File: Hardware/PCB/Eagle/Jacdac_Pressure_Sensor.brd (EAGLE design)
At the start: 27.9 x 27.9 mm, 29 parts, among them J1 JACDAC_EDGE_CONN-INNIE, J2 SWD-ADAPTER-, U1 NCP114ASN330T1G, U2 STM32F042F6P6, U3 LPS33HWTR, U4 BAT54S,235

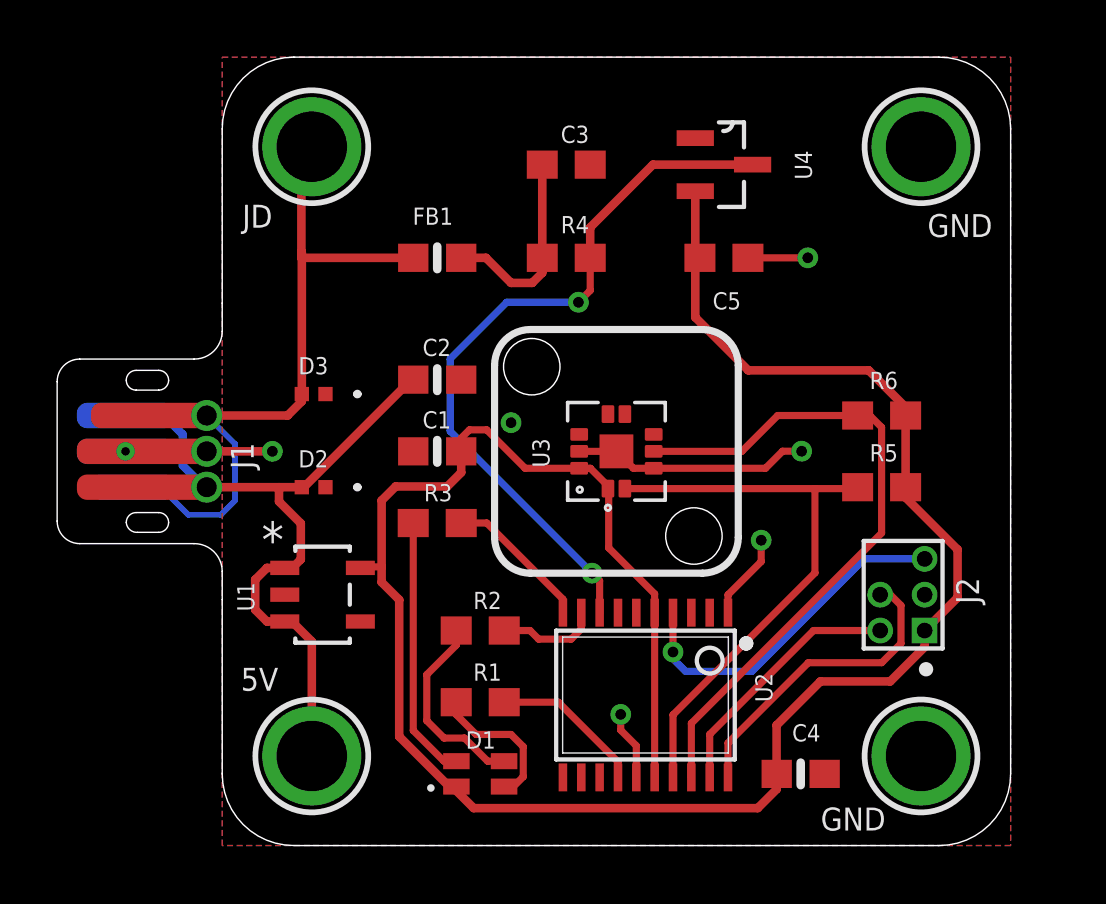
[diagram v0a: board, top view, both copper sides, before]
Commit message: Added version 1.0
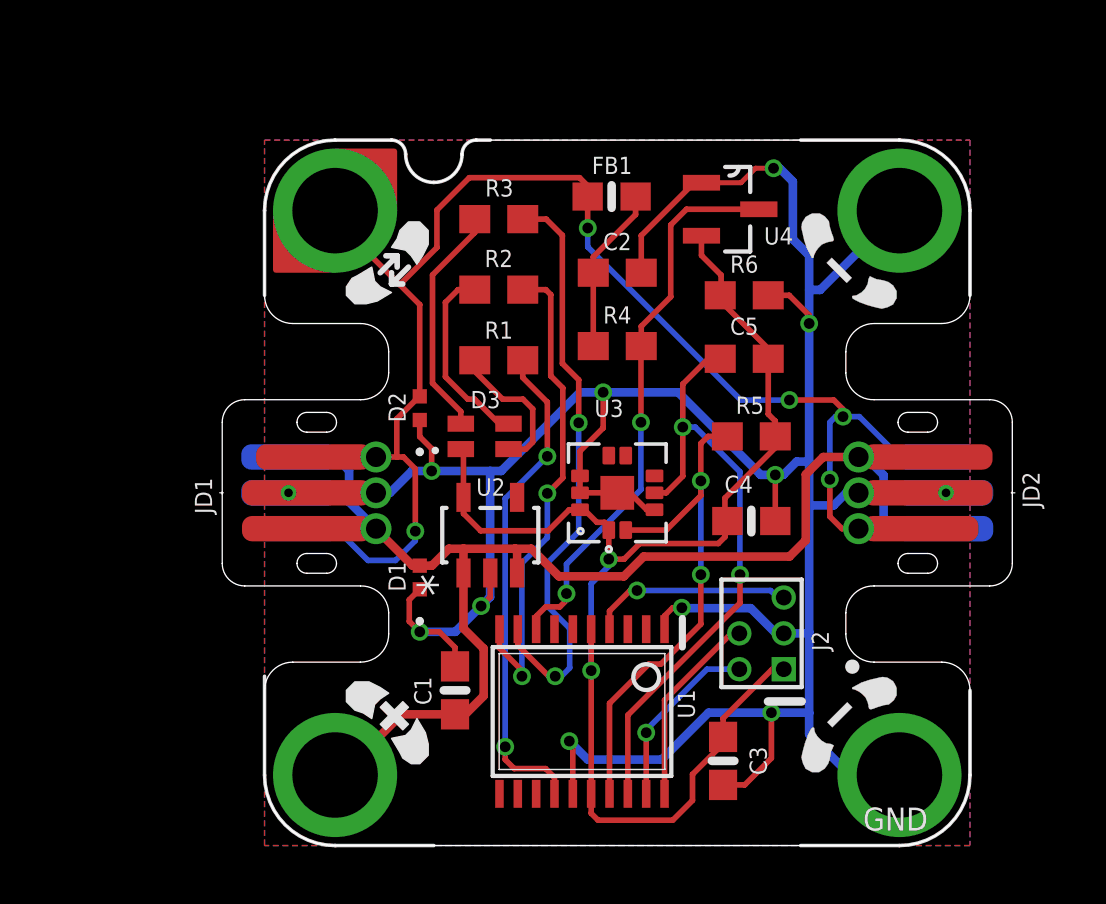
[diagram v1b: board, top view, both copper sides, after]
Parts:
- removed H1, H2, H3, H4: MOUNTINGHOLE2.5, milador:MOUNTINGHOLE_2.5_PLATED
- removed J1: JACDAC_EDGE_CONN-INNIE, Jacdac:JACDAC-EDGE-CONN-INNIE
- removed LABEL2: JACDAC-DEVICE-PS, milador:JACDAC-PRESSURE-SENSOR
- removed LABEL3: MILADOR-LOGO-, milador:MILADOR_LOGO1
- removed U$1: JACDAC-DEVICE-LPS33HW, milador:JACDAC-LPS33HW
- added J3: 5V, milador:M3-HOLE-PWR-OUTL
- added J4: DATA, milador:M3-HOLE-DATA-NOTCH
- added J5, J6: GND, milador:M3-HOLE-GND
- added JD1, JD2: JACDAC-EDGE-OUTIE, milador:JD-EDGE-OUTIE
- added LABEL_JACDAC_PS: MILADOR-JACDAC-DEVICE-PS, milador:JACDAC-PRESSURE-SENSOR
- added LABEL_LPS33HW: MILADOR-JACDAC-DEVICE-LPS33HW, milador:JACDAC-LPS33HW
- added LABEL_MILADOR: MILADOR-LOGO-, milador:MILADOR_LOGO1
- added LABEL_QR_CODE: MILADOR-QR-CODE-JACDAC-GITHUB-PS, milador:MILADOR_QR_JACDAC_PS
- C1: value 0.1uF -> 1uF
- C2: value 1uF -> 33pF; device milador_SMD:0603-NO -> milador_SMD:0603
- C3: value 33pF -> 1uF; device milador_SMD:0603 -> milador_SMD:0603-NO
- C4: value 1uF -> 0.1uF
- D1: value LED-HSMF-C114 -> DIODE-ZENER-AA-RCLAMP0521PATCT; device milador_SMD:DIOSC160X150X35-4N -> milador_SMD:DIODE-ZENER-0402
- D2: value RCLAMP0521PATCT -> DIODE-ZENER-AA-RCLAMP0521PATCT
- D3: value RCLAMP0521PATCT -> LED-HSMF-C114; device milador_SMD:DIODE-ZENER-0402 -> milador_SMD:DIOSC160X150X35-4N
- MMC_LOGO: value MMC_LOGO-SM -> MMC_LOGO-XSM; device MMC Eagle:MMC_SMALL_LOGO -> MMC Eagle:MMC_X-SMALL_LOGO
- U1: value NCP114ASN330T1G -> STM32F042F6P6; device milador_SMD:TSOP-5_ONS -> milador_SMD:TSSOP20
- U2: value STM32F042F6P6 -> NCP114ASN330T1G; device milador_SMD:TSSOP20 -> milador_SMD:TSOP-5_ONS
- moved C3 21.8 mm to (17.8, 3.00), turned to 270 degrees
- moved R1 12.1 mm to (9.80, 17.2)
- moved R2 12.1 mm to (9.80, 19.7)
- moved R3 11.0 mm to (9.80, 22.2)
- moved U1 10.1 mm to (12.8, 4.75), turned to 180 degrees
- moved MMC_LOGO 9.48 mm to (12.0, 4.50), turned to 0 degrees
- moved C4 9.13 mm to (18.8, 11.5)
- moved C1 8.49 mm to (8.25, 5.50), turned to 90 degrees
- moved U2 7.90 mm to (9.50, 11.0), turned to 90 degrees
- moved C2 7.42 mm to (14.0, 20.3)
- moved D1 7.28 mm to (7.00, 9.50), turned to 90 degrees
- moved FB1 6.55 mm to (13.8, 23.0)
- moved D3 6.24 mm to (9.30, 14.5), turned to 0 degrees
- moved R6 5.27 mm to (18.5, 17.2)
- moved J2 5.18 mm to (19.9, 6.25)
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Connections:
- net +3V3: now also C3.1, D3.1, U1.16; no longer C1.1, D1.1, U2.16
- net GND: now also D1.1, J5.H, J6.H, JD1.2, JD1.5, JD1.P$2, JD1.P$4, JD2.2, JD2.5, JD2.P$2, JD2.P$4, U1.1, U1.15, U2.2; no longer D3.1, H3.P$1, H4.P$1, J1.GND1, J1.GND2, J1.GND3, J1.GND4, U1.2, U2.1, U2.15
- net JD_DATA: now also U1.8; no longer U2.8
- net J_DATA: now also D2.2, J4.H, JD1.1, JD1.6, JD1.P$3, JD2.1, JD2.6, JD2.P$3; no longer D3.2, H2.P$1, J1.JD1, J1.JD2, J1.JD3
- net N$1: now also D3.4; no longer D1.4
- net N$2: now also D3.3; no longer D1.3
- net N$3: now also D3.2; no longer D1.2
- net N$4: now also C2.1; no longer C3.1
- net RESET: now also U1.4; no longer U2.4
- net RGB_B: now also U1.14; no longer U2.14
- net RGB_G: now also U1.10; no longer U2.9
- net RGB_R: now also U1.9; no longer U2.10
- net SCL: now also U1.17; no longer U2.17
- net SDA: now also U1.18; no longer U2.18
- net SWCLK: now also U1.20; no longer U2.20
- net SWDIO: now also U1.19; no longer U2.19
- net VCC: now also C1.1, D1.2, J3.H, JD1.3, JD1.4, JD1.P$1, JD2.3, JD2.4, JD2.P$1, U2.1, U2.3; no longer C2.1, D2.2, H1.P$1, J1.VDD1, J1.VDD2, J1.VDD3, U1.1, U1.3
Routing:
- net GND: track 21.4 -> 108.6 mm, vias 6 -> 10
- net +3V3: track 77.9 -> 47.4 mm, vias 0 -> 2
- net J_DATA: track 26.6 -> 51.4 mm, vias 0 -> 5
- net VCC: track 28.1 -> 48.9 mm
- net RGB_R: track 5.20 -> 21.0 mm, vias 0 -> 2
- net RGB_G: track 3.58 -> 17.4 mm, vias 0 -> 2
- net RGB_B: track 5.46 -> 17.7 mm, vias 0 -> 2
- net JD_DATA: track 26.1 -> 19.9 mm
- net RESET: track 12.4 -> 7.22 mm
- net SWCLK: track 11.0 -> 6.95 mm
- net SWDIO: track 9.09 -> 6.46 mm, vias 0 -> 1
- net SDA: track 24.0 -> 21.9 mm, vias 0 -> 2
- net SCL: track 20.6 -> 18.7 mm, vias 0 -> 2
- net N$4: track 7.22 -> 5.92 mm
- net N$3: track 9.33 -> 8.29 mm
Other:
- board size 27.9 x 27.9 mm -> 25 x 25 mm
- board text added: "V1.1"
- board text removed: "5V"
- board text removed: "JD"
